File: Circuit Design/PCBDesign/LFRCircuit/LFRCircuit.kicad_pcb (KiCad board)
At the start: 2 copper layers, 90 x 53.1 mm, 32 parts, among them J1 OLED_128x64, M1 Motor_DC, M2 Motor_DC, U1 L293D, U2 TPS54202DDC

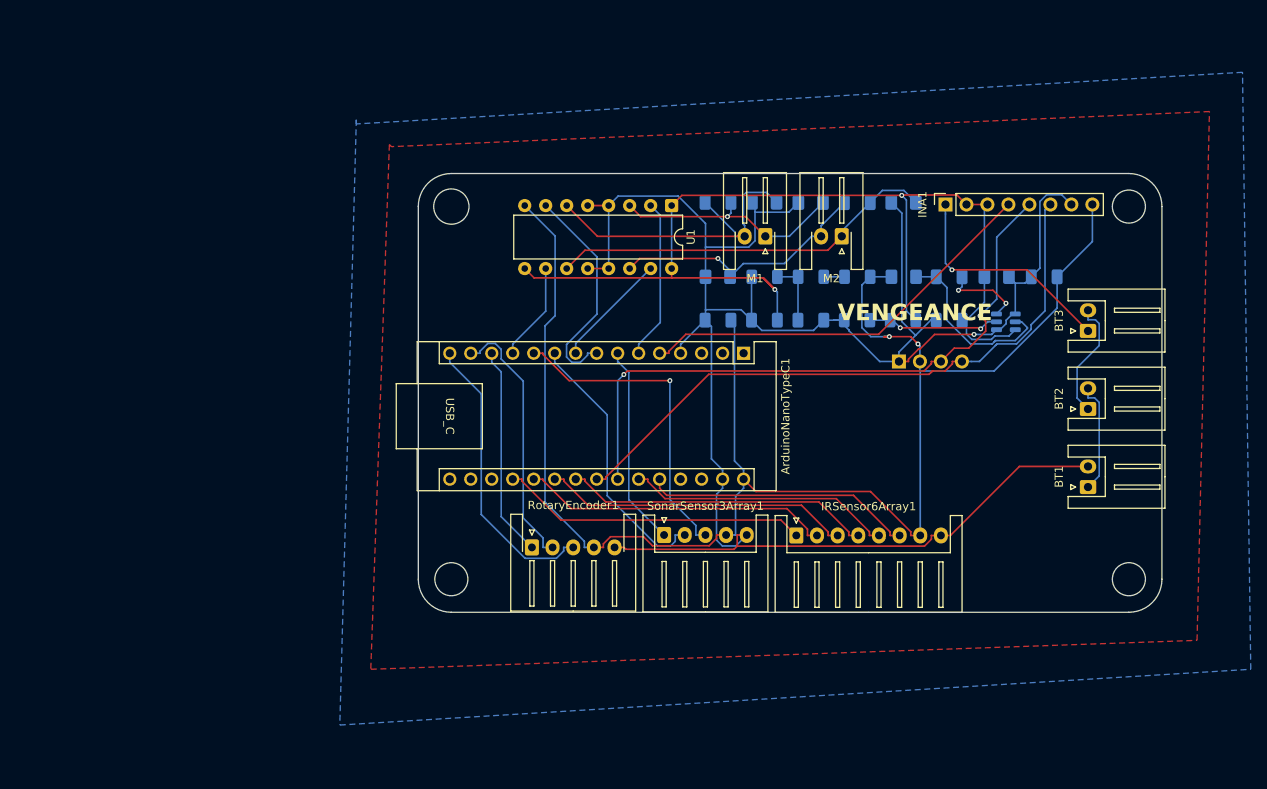
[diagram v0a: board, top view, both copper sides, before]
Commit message: Updated PCB
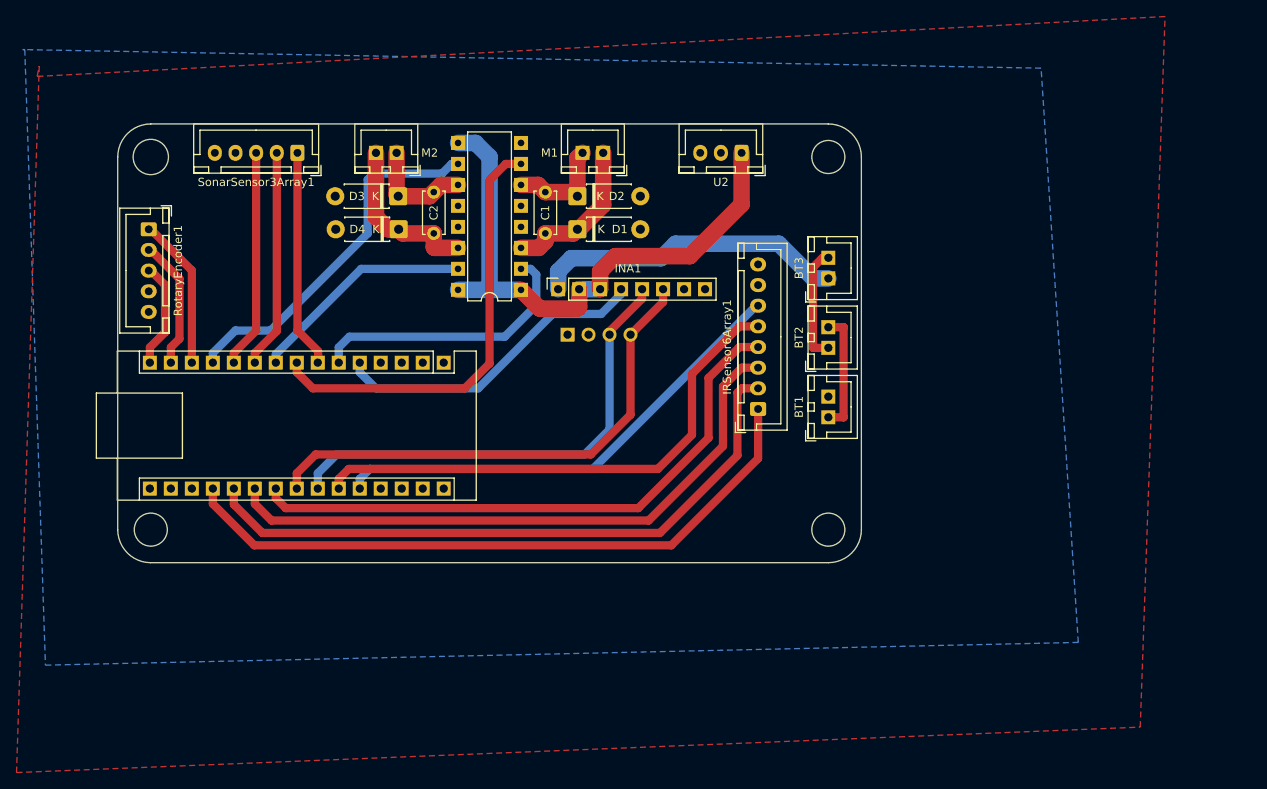
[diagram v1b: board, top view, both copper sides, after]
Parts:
- removed C3: 10uF, Capacitor_SMD:C_1206_3216Metric_Pad1.33x1.80mm_HandSolder
- removed C4, C5: 0.1uF, Capacitor_SMD:C_1206_3216Metric_Pad1.33x1.80mm_HandSolder
- removed C6, C7: 22uF, Capacitor_SMD:C_1206_3216Metric_Pad1.33x1.80mm_HandSolder
- removed C8: 75pF, Capacitor_SMD:C_1206_3216Metric_Pad1.33x1.80mm_HandSolder
- removed D5: D, Diode_SMD:D_1206_3216Metric_Pad1.42x1.75mm_HandSolder
- removed L1: 15uH, Inductor_SMD:L_1206_3216Metric_Pad1.42x1.75mm_HandSolder
- removed R1: 49.9, Resistor_SMD:R_1206_3216Metric_Pad1.30x1.75mm_HandSolder
- removed R2: 100K, Resistor_SMD:R_1206_3216Metric_Pad1.30x1.75mm_HandSolder
- removed R3: 13.3K, Resistor_SMD:R_1206_3216Metric_Pad1.30x1.75mm_HandSolder
- removed R4: 511K, Resistor_SMD:R_1206_3216Metric_Pad1.30x1.75mm_HandSolder
- removed R5: 105K, Resistor_SMD:R_1206_3216Metric_Pad1.30x1.75mm_HandSolder
- ArduinoNanoTypeC1: footprint ArduinoNano:ArduinoNanoTypeC -> RactangularPad:ArduinoNanoRactangularPads
- BT1, BT2, BT3: footprint Connector_JST:JST_XH_S2B-XH-A_1x02_P2.50mm_Horizontal -> RactangularPad:JST_XH_B2B-XH-A_1x02_P2.50mm_Vertical_ractangular
- C1, C2: footprint Capacitor_SMD:C_1206_3216Metric_Pad1.33x1.80mm_HandSolder -> Capacitor_THT:C_Disc_D5.0mm_W2.5mm_P5.00mm; moved to F.Cu
- D1, D2, D3, D4: footprint Diode_SMD:D_1206_3216Metric_Pad1.42x1.75mm_HandSolder -> Diode_THT:D_DO-41_SOD81_P7.62mm_Horizontal; moved to F.Cu
- INA1: footprint Connector_PinSocket_2.54mm:PinSocket_1x08_P2.54mm_Vertical -> RactangularPad:PinSocket_1x08_P2.54mm_Vertical_ractangular
- IRSensor6Array1: footprint Connector_JST:JST_XH_S8B-XH-A_1x08_P2.50mm_Horizontal -> Connector_JST:JST_XH_B8B-XH-A_1x08_P2.50mm_Vertical
- M1, M2: footprint Connector_JST:JST_XH_S2B-XH-A-1_1x02_P2.50mm_Horizontal -> RactangularPad:JST_XH_B2B-XH-A_1x02_P2.50mm_Vertical_ractangular
- RotaryEncoder1: footprint Connector_JST:JST_XH_S5B-XH-A-1_1x05_P2.50mm_Horizontal -> Connector_JST:JST_XH_B5B-XH-A_1x05_P2.50mm_Vertical
- SonarSensor3Array1: footprint Connector_JST:JST_XH_S5B-XH-A_1x05_P2.50mm_Horizontal -> Connector_JST:JST_XH_B5B-XH-A_1x05_P2.50mm_Vertical
- U1: footprint Package_DIP:DIP-16_W7.62mm -> RactangularPad:DIP-16_W7.62mm_ractangularPads
- U2: value TPS54202DDC -> ~; footprint Package_TO_SOT_SMD:SOT-23-6 -> Connector_JST:JST_XH_B3B-XH-A_1x03_P2.50mm_Vertical; moved to F.Cu
- moved SonarSensor3Array1 64.1 mm to (110.9, 72.0), turned to 180 degrees
- moved D3 61.2 mm to (123.1, 77.2)
- moved RotaryEncoder1 60.3 mm to (92.9, 81.2), turned to -90 degrees
- moved M2 54.8 mm to (122.9, 72.0)
- moved C2 51.3 mm to (127.4, 76.8), turned to -90 degrees
- moved INA1 48.0 mm to (142.4, 88.5)
- moved J1 40.2 mm to (147.4, 94.0)
- moved D4 39.1 mm to (123.1, 81.2)
- moved U2 38.0 mm to (164.6, 72.0)
- moved ArduinoNanoTypeC1 36.3 mm to (128.6, 97.4)
- moved BT1 32.5 mm to (175.1, 104.0)
- moved BT2 32.3 mm to (175.1, 95.6)
- moved BT3 32.1 mm to (175.1, 87.2)
- moved D1 28.4 mm to (144.8, 81.2), turned to 0 degrees
- moved D2 22.6 mm to (144.8, 77.2), turned to 0 degrees
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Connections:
- ArduinoNanoTypeC1 pad 29: GND -> unconnected-(ArduinoNanoTypeC1-GND-Pad29)
- U2 pad 1: GND -> +12V
- U2 pad 2: Net-(U2-SW) -> GND
- U2 pad 3: +12V -> +5V
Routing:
- net GND: track 253.5 -> 0.00 mm, vias 1 -> 0
- net +5V: track 195.4 -> 0.00 mm, vias 2 -> 0
- net +12V: track 130.8 -> 69.7 mm, vias 2 -> 0
- net /IR1: track 37.3 -> 80.3 mm
- net /IR2: track 37.6 -> 78.5 mm
- net /IR3: track 37.4 -> 75.5 mm
- net /IR4: track 37.4 -> 72.7 mm
- net Net-(D3-K): track 47.2 -> 13.1 mm
- net /M2B: track 11.9 -> 44.1 mm
- net /IR5: track 32.3 -> 63.9 mm
- net Net-(D2-K): track 39.5 -> 12.9 mm
- net /M1B: track 26.9 -> 53.4 mm
- net /IR6: track 32.8 -> 58.1 mm
- net /RE_SW: track 35.2 -> 13.1 mm
- net Net-(U2-SW): track 22.0 -> 0.00 mm
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- added copper zone on B.Cu, net +5V
- added copper zone on F.Cu, net GND
- removed copper zone on F.Cu, net +12V
- removed copper zone on B.Cu, net GND
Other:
- board text removed: "VENGEANCE"
